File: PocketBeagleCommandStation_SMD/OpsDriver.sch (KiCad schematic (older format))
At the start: 0 parts

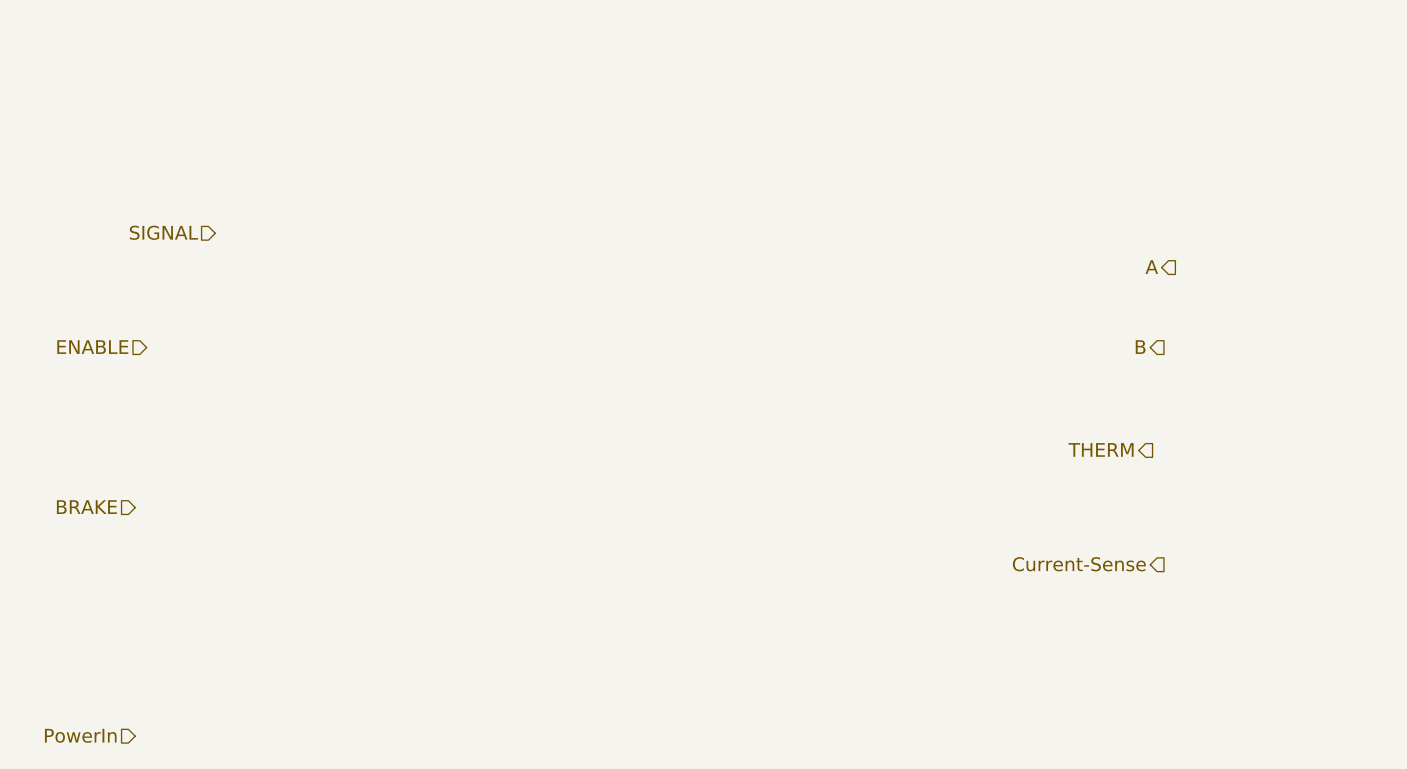
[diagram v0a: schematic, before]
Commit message: Working on PocketBeagleCommandStation_SMD.
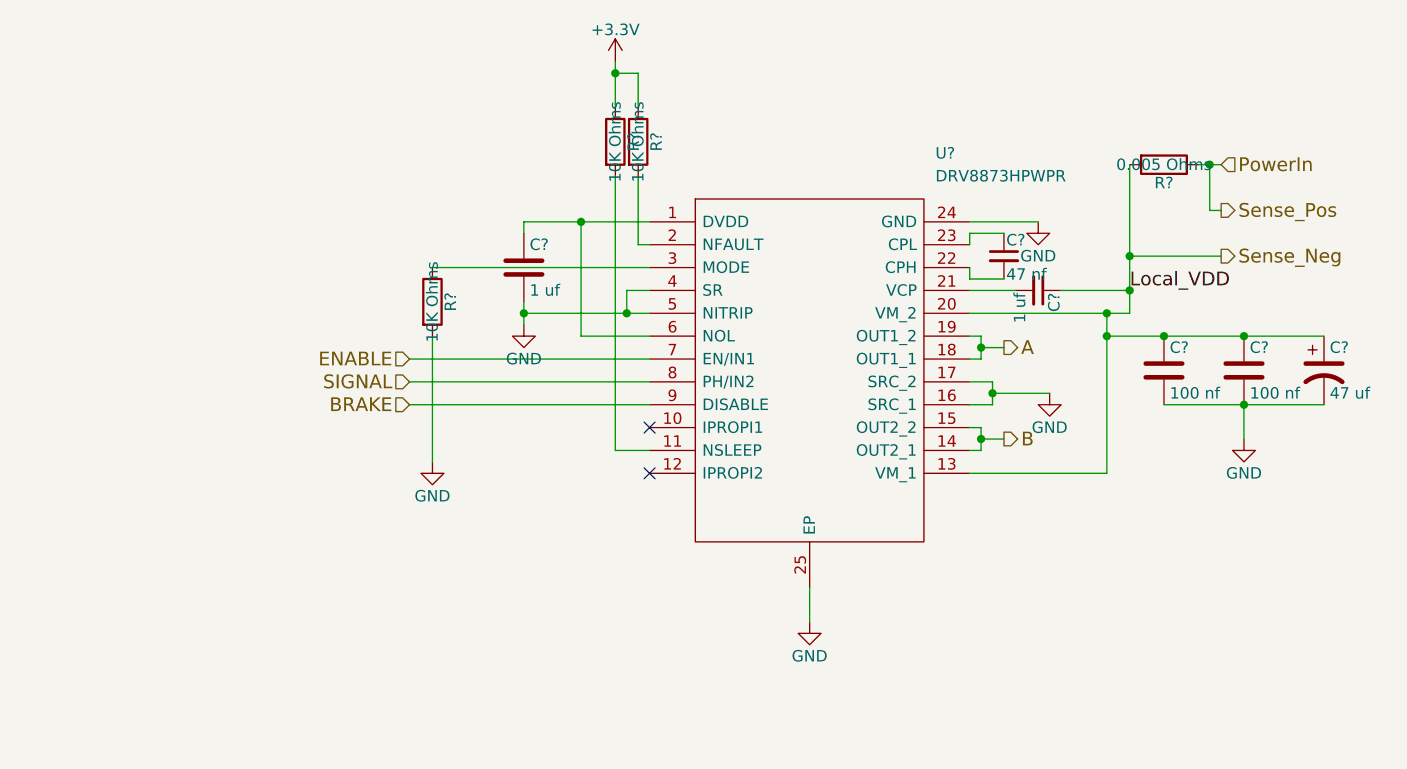
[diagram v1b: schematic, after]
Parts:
- added C?: 47 nf, symbol C_Small
- added C?: 1 uf, symbol C_Small
- added C? (x2): 100 nf, symbol C
- added C?: 47 uf, symbol CP1
- added C?: 1 uf, symbol C
- added R?: 0.005 Ohms, symbol R
- added R? (x3): 10K Ohms, symbol R
- added U?: DRV8873HPWPR, SOP65P640X120-25N, symbol DRV8873HPWPR
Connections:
- net A: now also U?.18 (OUT1_1), U?.19 (OUT1_2)
- net B: now also U?.14 (OUT2_1), U?.15 (OUT2_2)
- net BRAKE: now also U?.9 (DISABLE)
- net ENABLE: now also U?.7 (EN/IN1)
- net PowerIn: now also R?.1
- net SIGNAL: now also U?.8 (PH/IN2)
- new net: C?.1, U?.1 (DVDD), U?.6 (NOL)
- new net: R?.2, U?.11 (NSLEEP)
- new net: R?.2, U?.2 (NFAULT)
- new net: C?.2, U?.21 (VCP)
- new net: C?.2, U?.22 (CPH)
- new net: C?.1, U?.23 (CPL)
- new net: R?.1, U?.3 (MODE)
- new net +3V3: R?.1, R?.1
- new net GND: C?.2, C?.2, C?.2, C?.2, R?.2, U?.16 (SRC_1), U?.17 (SRC_2), U?.24 (GND), U?.25 (EP), U?.4 (SR), U?.5 (NITRIP)
- new net Sense_Neg: C?.1, C?.1, C?.1, C?.1, R?.2, U?.13 (VM_1), U?.20 (VM_2)
- no-connect marks 0 -> 2

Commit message: Continuing work on PocketBeagleCommandStation_SMD.
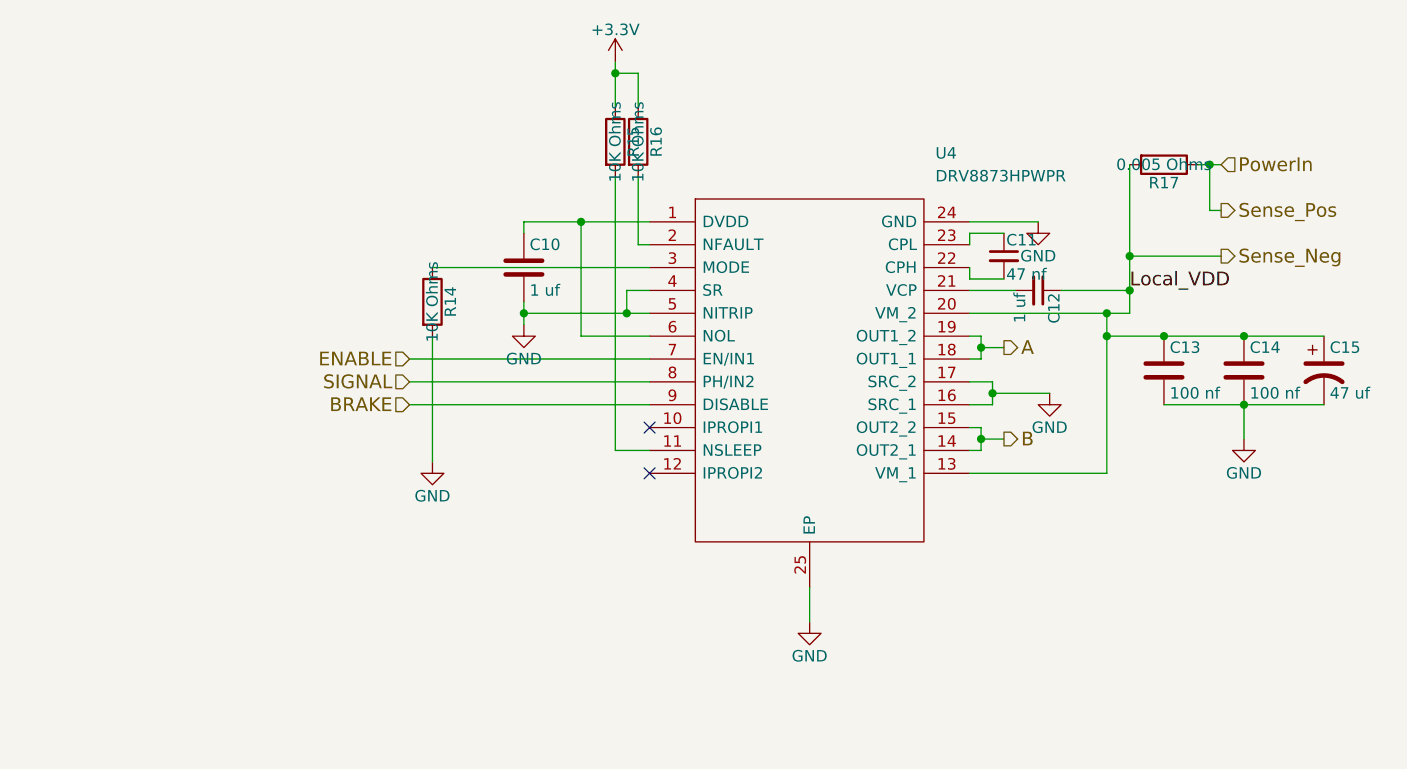
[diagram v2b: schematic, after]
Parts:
- U4: renamed from U?; footprint SOP65P640X120-25N -> SOP65P640X120:SOP65P640X120-25N
- gave numbers to parts that had none: 10
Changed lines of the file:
@@
 LIBS:DRV8873HPWPR
 LIBS:DRV8801PWP
+LIBS:74ahc1g08
+LIBS:mcp9701at
 LIBS:PocketBeagleCommandStation_SMD-cache
 EELAYER 25 0
@@
 Sense_Neg
 $Comp
-L DRV8873HPWPR U?
+L DRV8873HPWPR U4
 U 1 1 606FD60F
 P 3550 1800
-F 0 "U?" H 4800 2100 50  0000 L CNN
+F 0 "U4" H 4800 2100 50  0000 L CNN
 F 1 "DRV8873HPWPR" H 4800 2000 50  0000 L CNN
-F 2 "SOP65P640X120-25N" H 4800 1900 50  0001 L CNN
+F 2 "SOP65P640X120:SOP65P640X120-25N" H 4800 1900 50  0001 L CNN
 F 3 "http://www.ti.com/lit/ds/symlink/drv8873.pdf" H 4800 1800 50  0001 L CNN
 F 4 "Motor / Motion / Ignition Controllers & Drivers 10A H-Bridge Motor Driver with Integrated Current Sensing and Current Sense Output" H 4800 1700 50  0001 L CNN "Description"
@@
 $EndComp
 $Comp
-L GND #PWR?
+L GND #PWR028
 U 1 1 6070432B
 P 5250 1800
-F 0 "#PWR?" H 5250 1550 50  0001 C CNN
+F 0 "#PWR028" H 5250 1550 50  0001 C CNN
 F 1 "GND" H 5250 1650 50  0000 C CNN
 F 2 "" H 5250 1800 50  0001 C CNN
@@
 $EndComp
 $Comp
-L GND #PWR?
+L GND #PWR029
 U 1 1 60704370
 P 4250 3550
-F 0 "#PWR?" H 4250 3300 50  0001 C CNN
+F 0 "#PWR029" H 4250 3300 50  0001 C CNN
 F 1 "GND" H 4250 3400 50  0000 C CNN
 F 2 "" H 4250 3550 50  0001 C CNN
@@
 $EndComp
 $Comp
-L R R?
+L R R17
 U 1 1 607043BF
 P 5800 1550
-F 0 "R?" V 5880 1550 50  0000 C CNN
+F 0 "R17" V 5880 1550 50  0000 C CNN
 F 1 "0.005 Ohms" V 5800 1550 50  0000 C CNN
 F 2 "" V 5730 1550 50  0001 C CNN
@@
 Local_VDD
 $Comp
-L C_Small C?
+L C_Small C11
 U 1 1 607044D9
 P 5100 1950
-F 0 "C?" H 5110 2020 50  0000 L CNN
+F 0 "C11" H 5110 2020 50  0000 L CNN
 F 1 "47 nf" H 5110 1870 50  0000 L CNN
 F 2 "" H 5100 1950 50  0001 C CNN
@@
 $EndComp
 $Comp
-L C_Small C?
+L C_Small C12
 U 1 1 6070454C
 P 5250 2100
-F 0 "C?" H 5260 2170 50  0000 L CNN
+F 0 "C12" H 5260 2170 50  0000 L CNN
 F 1 "1 uf" H 5260 2020 50  0000 L CNN
 F 2 "" H 5250 2100 50  0001 C CNN
@@
 $EndComp
 $Comp
-L C C?
+L C C13
 U 1 1 607045D9
 P 5800 2450
-F 0 "C?" H 5825 2550 50  0000 L CNN
+F 0 "C13" H 5825 2550 50  0000 L CNN
 F 1 "100 nf" H 5825 2350 50  0000 L CNN
 F 2 "" H 5838 2300 50  0001 C CNN
@@
 $EndComp
 $Comp
-L C C?
+L C C14
 U 1 1 607045FC
 P 6150 2450
-F 0 "C?" H 6175 2550 50  0000 L CNN
+F 0 "C14" H 6175 2550 50  0000 L CNN
 F 1 "100 nf" H 6175 2350 50  0000 L CNN
 F 2 "" H 6188 2300 50  0001 C CNN
@@
 $EndComp
 $Comp
-L CP1 C?
+L CP1 C15
 U 1 1 60704621
 P 6500 2450
-F 0 "C?" H 6525 2550 50  0000 L CNN
+F 0 "C15" H 6525 2550 50  0000 L CNN
 F 1 "47 uf" H 6525 2350 50  0000 L CNN
 F 2 "" H 6500 2450 50  0001 C CNN
@@
 $EndComp
 $Comp
-L GND #PWR?
+L GND #PWR030
 U 1 1 60704783
 P 6150 2750
-F 0 "#PWR?" H 6150 2500 50  0001 C CNN
+F 0 "#PWR030" H 6150 2500 50  0001 C CNN
 F 1 "GND" H 6150 2600 50  0000 C CNN
 F 2 "" H 6150 2750 50  0001 C CNN
@@
 $EndComp
 $Comp
-L GND #PWR?
+L GND #PWR031
 U 1 1 60704831
 P 5300 2550
-F 0 "#PWR?" H 5300 2300 50  0001 C CNN
+F 0 "#PWR031" H 5300 2300 50  0001 C CNN
 F 1 "GND" H 5300 2400 50  0000 C CNN
 F 2 "" H 5300 2550 50  0001 C CNN
@@
 NoConn ~ 3550 2900
 $Comp
-L C C?
+L C C10
 U 1 1 607048DD
 P 3000 2000
-F 0 "C?" H 3025 2100 50  0000 L CNN
+F 0 "C10" H 3025 2100 50  0000 L CNN
 F 1 "1 uf" H 3025 1900 50  0000 L CNN
 F 2 "" H 3038 1850 50  0001 C CNN
@@
 $EndComp
 $Comp
-L GND #PWR?
+L GND #PWR032
 U 1 1 6070495B
 P 3000 2250
-F 0 "#PWR?" H 3000 2000 50  0001 C CNN
+F 0 "#PWR032" H 3000 2000 50  0001 C CNN
 F 1 "GND" H 3000 2100 50  0000 C CNN
 F 2 "" H 3000 2250 50  0001 C CNN
@@
 $EndComp
 $Comp
-L R R?
+L R R16
 U 1 1 60704A49
 P 3500 1450
-F 0 "R?" V 3580 1450 50  0000 C CNN
+F 0 "R16" V 3580 1450 50  0000 C CNN
 F 1 "10K Ohms" V 3500 1450 50  0000 C CNN
 F 2 "" V 3430 1450 50  0001 C CNN
@@
 $EndComp
 $Comp
-L R R?
+L R R15
 U 1 1 60704A7E
 P 3400 1450
-F 0 "R?" V 3480 1450 50  0000 C CNN
+F 0 "R15" V 3480 1450 50  0000 C CNN
 F 1 "10K Ohms" V 3400 1450 50  0000 C CNN
 F 2 "" V 3330 1450 50  0001 C CNN
@@
 $EndComp
 $Comp
-L +3.3V #PWR?
+L +3.3V #PWR033
 U 1 1 60707495
 P 3400 1100
-F 0 "#PWR?" H 3400 950 50  0001 C CNN
+F 0 "#PWR033" H 3400 950 50  0001 C CNN
 F 1 "+3.3V" H 3400 1240 50  0000 C CNN
 F 2 "" H 3400 1100 50  0001 C CNN
@@
 $EndComp
 $Comp
-L R R?
+L R R14
 U 1 1 6070758B
 P 2600 2150
-F 0 "R?" V 2680 2150 50  0000 C CNN
+F 0 "R14" V 2680 2150 50  0000 C CNN
 F 1 "10K Ohms" V 2600 2150 50  0000 C CNN
 F 2 "" V 2530 2150 50  0001 C CNN
@@
 $EndComp
 $Comp
-L GND #PWR?
+L GND #PWR034
 U 1 1 607075FE
 P 2600 2850
-F 0 "#PWR?" H 2600 2600 50  0001 C CNN
+F 0 "#PWR034" H 2600 2600 50  0001 C CNN
 F 1 "GND" H 2600 2700 50  0000 C CNN
 F 2 "" H 2600 2850 50  0001 C CNN
@@
 	5100 2350 5000 2350
 Wire Wire Line
-	5000 2300 5000 2350
-Wire Wire Line
-	5000 2350 5000 2400
+	5000 2300 5000 2400
 Wire Wire Line
 	5000 2300 4950 2300
@@
 	5100 2750 5000 2750
 Wire Wire Line
-	5000 2700 5000 2750
-Wire Wire Line
-	5000 2750 5000 2800
+	5000 2700 5000 2800
 Wire Wire Line
 	5000 2700 4950 2700
@@
 Connection ~ 5000 2750
 Wire Wire Line
-	4950 2200 5550 2200
-Wire Wire Line
-	5550 2200 5650 2200
-Wire Wire Line
-	5550 2200 5550 2300
-Wire Wire Line
-	5550 2300 5550 2900
+	5650 2200 4950 2200
+Wire Wire Line
+	5550 2200 5550 2900
 Wire Wire Line
 	5550 2900 4950 2900
@@
 	4250 3400 4250 3550
 Wire Wire Line
-	6050 1550 6000 1550
-Wire Wire Line
-	6000 1550 5950 1550
-Wire Wire Line
-	5650 2200 5650 2100
-Wire Wire Line
-	5650 2100 5650 1950
-Wire Wire Line
-	5650 1950 5650 1550
+	5950 1550 6050 1550
+Wire Wire Line
+	5650 1550 5650 2200
 Connection ~ 5550 2200
 Wire Wire Line
@@
 Connection ~ 5650 2100
 Wire Wire Line
-	5550 2300 5800 2300
-Wire Wire Line
-	5800 2300 6150 2300
-Wire Wire Line
-	6150 2300 6500 2300
+	5550 2300 6500 2300
 Connection ~ 6150 2300
 Connection ~ 5550 2300
 Connection ~ 5800 2300
 Wire Wire Line
-	5800 2600 6150 2600
-Wire Wire Line
-	6150 2600 6500 2600
+	5800 2600 6500 2600
 Connection ~ 6150 2600
 Wire Wire Line
@@
 	4950 2500 5050 2500
 Wire Wire Line
-	5050 2500 5050 2550
-Wire Wire Line
-	5050 2550 5050 2600
+	5050 2500 5050 2600
 Wire Wire Line
 	5050 2600 4950 2600
@@
 Connection ~ 5050 2550
 Wire Wire Line
-	3000 1800 3250 1800
-Wire Wire Line
-	3250 1800 3550 1800
+	3000 1800 3550 1800
 Wire Wire Line
 	3250 1800 3250 2300
@@
 Connection ~ 3250 1800
 Wire Wire Line
-	3000 2150 3000 2200
-Wire Wire Line
-	3000 2200 3000 2250
+	3000 2150 3000 2250
 Wire Wire Line
 	3500 1600 3500 1900
@@
 	3400 2800 3550 2800
 Wire Wire Line
-	3400 1100 3400 1150
-Wire Wire Line
-	3400 1150 3400 1300
+	3400 1100 3400 1300
 Wire Wire Line
 	3500 1300 3500 1150
@@
 	3450 2100 3450 2200
 Wire Wire Line
-	3000 2200 3450 2200
-Wire Wire Line
-	3450 2200 3550 2200
+	3000 2200 3550 2200
 Connection ~ 3000 2200
 Connection ~ 3450 2200
